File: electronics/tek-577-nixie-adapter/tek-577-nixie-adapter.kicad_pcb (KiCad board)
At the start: 2 copper layers, 31.7 x 61 mm, 6 parts, among them J1 C, J2 Conn_01x11_Socket, J3 E

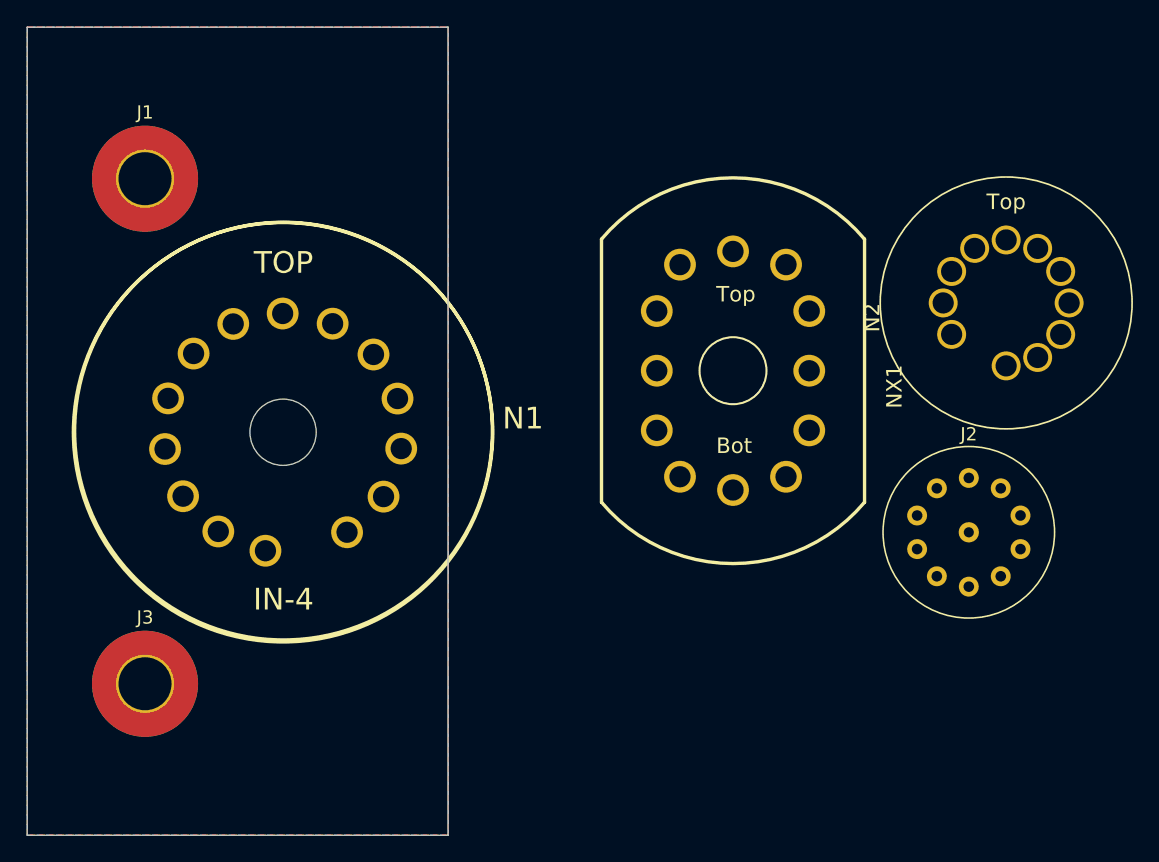
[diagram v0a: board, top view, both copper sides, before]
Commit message: board design done
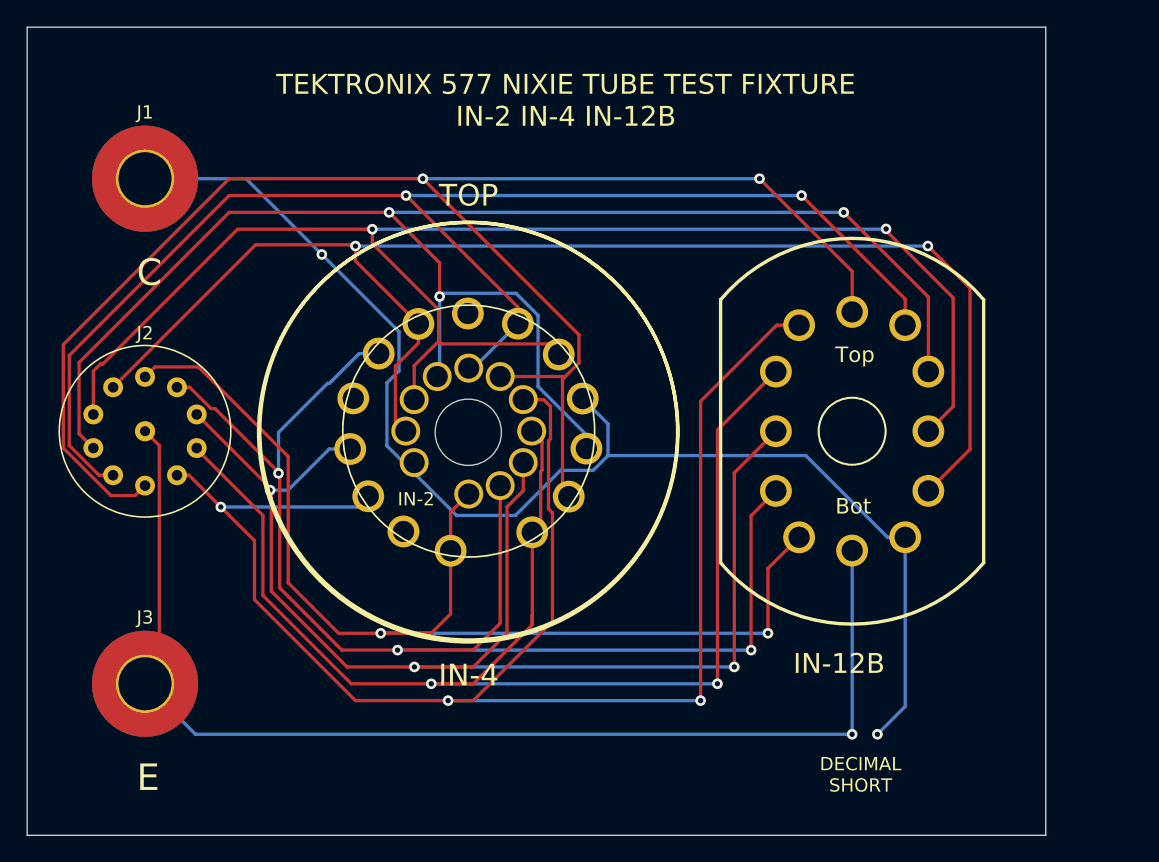
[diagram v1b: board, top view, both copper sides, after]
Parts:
- moved J2 62.6 mm to (134.6, 94.0)
- moved N2 41.7 mm to (159.0, 94.0)
- moved N1 14.0 mm to (159.0, 94.0)
- moved NX1 10.1 mm to (188.0, 94.0)
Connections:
- NX1 pad LHDP: unconnected-(NX1-PadLHDP) -> /E
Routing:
- net /5: track 0.00 -> 122.0 mm, vias 0 -> 3
- net /6: track 0.00 -> 120.9 mm, vias 0 -> 2
- net /8: track 0.00 -> 117.7 mm, vias 0 -> 3
- net /9: track 0.00 -> 110.8 mm, vias 0 -> 2
- net /0: track 0.00 -> 104.0 mm, vias 0 -> 2
- net /7: track 0.00 -> 102.5 mm, vias 0 -> 2
- net /2: track 0.00 -> 101.4 mm, vias 0 -> 3
- net /4: track 0.00 -> 101.0 mm, vias 0 -> 2
- net /3: track 0.00 -> 100.8 mm, vias 0 -> 3
- net /C: track 0.00 -> 99.9 mm, vias 0 -> 2
- net /E: track 0.00 -> 88.7 mm, vias 0 -> 1
- net /1: track 0.00 -> 84.9 mm, vias 0 -> 2
- removed copper zone on B.Cu, net (none)
- removed copper zone on F.Cu, net (none)
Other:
- board size 31.7 x 61 mm -> 76.8 x 61 mm
- board text added: "C"
- board text added: "DECIMAL SHORT"
- board text added: "E"
- board text added: "IN-12B"
- board text added: "IN-2"
- board text added: "TEKTRONIX 577 NIXIE TUBE TEST FIXTURE IN-2 IN-4 IN-12B"

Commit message: routing improvements
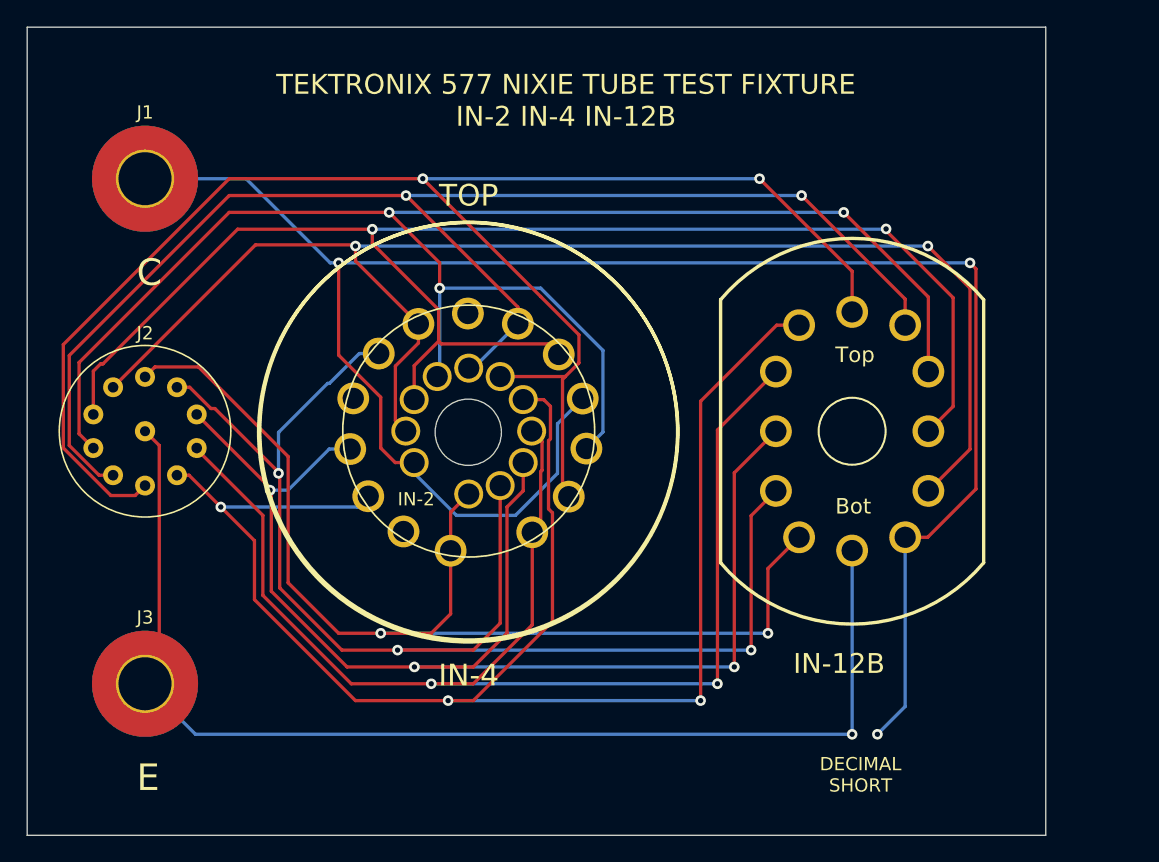
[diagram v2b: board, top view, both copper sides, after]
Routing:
- net /C: track 99.9 -> 143.6 mm, vias 2 -> 3
- net /8: track 117.7 -> 120.2 mm
- net /4: track 101.0 -> 100.3 mm
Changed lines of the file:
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@@
     (effects (font (size 2 2) (thickness 0.15)) (justify left bottom))
   )
+  (segment (start 152.4 95.25) (end 153.493357 96.343357) (width 0.25) (layer "F.Cu") (net 1))
+  (segment (start 149.225 88.239915) (end 152.4 91.414915) (width 0.25) (layer "F.Cu") (net 1))
+  (segment (start 196.85 81.28) (end 197.3 81.73) (width 0.25) (layer "F.Cu") (net 1))
+  (segment (start 153.493357 96.343357) (end 154.92327 96.343357) (width 0.25) (layer "F.Cu") (net 1))
+  (segment (start 149.225 81.28) (end 149.225 88.239915) (width 0.25) (layer "F.Cu") (net 1))
+  (segment (start 193.657056 101.98) (end 191.96 101.98) (width 0.25) (layer "F.Cu") (net 1))
+  (segment (start 197.3 98.337056) (end 193.657056 101.98) (width 0.25) (layer "F.Cu") (net 1))
+  (segment (start 197.3 81.73) (end 197.3 98.337056) (width 0.25) (layer "F.Cu") (net 1))
+  (segment (start 152.4 91.414915) (end 152.4 95.25) (width 0.25) (layer "F.Cu") (net 1))
   (via (at 189.865 116.84) (size 0.8) (drill 0.4) (layers "F.Cu" "B.Cu") (net 1))
-  (via (at 147.955 80.645) (size 0.8) (drill 0.4) (layers "F.Cu" "B.Cu") (net 1))
+  (via (at 149.225 81.28) (size 0.8) (drill 0.4) (layers "F.Cu" "B.Cu") (net 1))
+  (via (at 196.85 81.28) (size 0.8) (drill 0.4) (layers "F.Cu" "B.Cu") (net 1))
   (segment (start 191.96 114.745) (end 189.865 116.84) (width 0.25) (layer "B.Cu") (net 1))
+  (segment (start 154.92327 96.343357) (end 154.92327 97.13827) (width 0.25) (layer "B.Cu") (net 1))
+  (segment (start 165.735 93.417085) (end 167.637403 91.514682) (width 0.25) (layer "B.Cu") (net 1))
+  (segment (start 149.225 81.28) (end 148.59 81.28) (width 0.25) (layer "B.Cu") (net 1))
+  (segment (start 162.56 100.33) (end 165.735 97.155) (width 0.25) (layer "B.Cu") (net 1))
+  (segment (start 191.96 101.98) (end 191.96 114.745) (width 0.25) (layer "B.Cu") (net 1))
   (segment (start 154.92327 97.13827) (end 158.115 100.33) (width 0.25) (layer "B.Cu") (net 1))
-  (segment (start 153.778082 89.426918) (end 152.869716 90.335284) (width 0.25) (layer "B.Cu") (net 1))
-  (segment (start 147.955 80.645) (end 153.778082 86.468082) (width 0.25) (layer "B.Cu") (net 1))
-  (segment (start 162.56 100.33) (end 165.959619 96.930381) (width 0.25) (layer "B.Cu") (net 1))
-  (segment (start 169.545 95.816308) (end 169.545 93.422279) (width 0.25) (layer "B.Cu") (net 1))
-  (segment (start 154.92327 96.343357) (end 154.92327 97.13827) (width 0.25) (layer "B.Cu") (net 1))
-  (segment (start 154.128357 96.343357) (end 154.92327 96.343357) (width 0.25) (layer "B.Cu") (net 1))
-  (segment (start 142.24 74.93) (end 147.955 80.645) (width 0.25) (layer "B.Cu") (net 1))
-  (segment (start 169.545 95.816308) (end 184.469646 95.816308) (width 0.25) (layer "B.Cu") (net 1))
+  (segment (start 165.735 97.155) (end 165.735 93.417085) (width 0.25) (layer "B.Cu") (net 1))
   (segment (start 158.115 100.33) (end 162.56 100.33) (width 0.25) (layer "B.Cu") (net 1))
-  (segment (start 169.545 93.422279) (end 167.637403 91.514682) (width 0.25) (layer "B.Cu") (net 1))
-  (segment (start 168.430927 96.930381) (end 169.545 95.816308) (width 0.25) (layer "B.Cu") (net 1))
-  (segment (start 152.869716 95.084716) (end 154.128357 96.343357) (width 0.25) (layer "B.Cu") (net 1))
-  (segment (start 191.96 101.98) (end 191.96 114.745) (width 0.25) (layer "B.Cu") (net 1))
-  (segment (start 134.62 74.93) (end 142.24 74.93) (width 0.25) (layer "B.Cu") (net 1))
-  (segment (start 153.778082 86.468082) (end 153.778082 89.426918) (width 0.25) (layer "B.Cu") (net 1))
-  (segment (start 184.469646 95.816308) (end 190.633338 101.98) (width 0.25) (layer "B.Cu") (net 1))
-  (segment (start 165.959619 96.930381) (end 168.430927 96.930381) (width 0.25) (layer "B.Cu") (net 1))
-  (segment (start 152.869716 90.335284) (end 152.869716 95.084716) (width 0.25) (layer "B.Cu") (net 1))
-  (segment (start 190.633338 101.98) (end 191.96 101.98) (width 0.25) (layer "B.Cu") (net 1))
+  (segment (start 149.225 81.28) (end 196.85 81.28) (width 0.25) (layer "B.Cu") (net 1))
+  (segment (start 148.59 81.28) (end 142.24 74.93) (width 0.25) (layer "B.Cu") (net 1))
+  (segment (start 142.24 74.93) (end 134.62 74.93) (width 0.25) (layer "B.Cu") (net 1))
   (segment (start 135.695 95.055) (end 134.62 93.98) (width 0.25) (layer "F.Cu") (net 2))
   (segment (start 134.62 113.03) (end 135.695 111.955) (width 0.25) (layer "F.Cu") (net 2))
@@
   (segment (start 177.8 93.89) (end 182.21 89.48) (width 0.25) (layer "F.Cu") (net 6))
   (segment (start 164.567362 96.930381) (end 164.567362 94.749303) (width 0.25) (layer "F.Cu") (net 6))
-  (segment (start 163.83 108.585) (end 163.83 107.86) (width 0.25) (layer "F.Cu") (net 6))
   (segment (start 159.385 113.03) (end 163.83 108.585) (width 0.25) (layer "F.Cu") (net 6))
   (segment (start 143.51 100.33) (end 138.519331 95.339331) (width 0.25) (layer "F.Cu") (net 6))
@@
   (segment (start 159.39156 89.218657) (end 159.036716 89.218657) (width 0.25) (layer "B.Cu") (net 9))
   (segment (start 193.71 83.855) (end 193.71 89.48) (width 0.25) (layer "F.Cu") (net 10))
+  (segment (start 156.845 81.28) (end 153.035 77.47) (width 0.25) (layer "F.Cu") (net 10))
   (segment (start 187.325 77.47) (end 193.71 83.855) (width 0.25) (layer "F.Cu") (net 10))
   (segment (start 129.645669 88.792935) (end 129.645669 94.171969) (width 0.25) (layer "F.Cu") (net 10))
@@
   (segment (start 153.035 77.47) (end 140.968604 77.47) (width 0.25) (layer "F.Cu") (net 10))
   (segment (start 140.968604 77.47) (end 129.645669 88.792935) (width 0.25) (layer "F.Cu") (net 10))
-  (segment (start 156.845 81.28) (end 156.845 83.82) (width 0.25) (layer "F.Cu") (net 10))
-  (segment (start 153.035 77.47) (end 156.845 81.28) (width 0.25) (layer "F.Cu") (net 10))
+  (segment (start 156.845 83.185) (end 156.845 81.28) (width 0.25) (layer "F.Cu") (net 10))
   (via (at 187.325 77.47) (size 0.8) (drill 0.4) (layers "F.Cu" "B.Cu") (net 10))
   (via (at 153.035 77.47) (size 0.8) (drill 0.4) (layers "F.Cu" "B.Cu") (net 10))
-  (via (at 156.845 83.82) (size 0.8) (drill 0.4) (layers "F.Cu" "B.Cu") (net 10))
-  (segment (start 162.608478 83.574807) (end 164.268606 85.234935) (width 0.25) (layer "B.Cu") (net 10))
-  (segment (start 164.268606 85.234935) (end 164.268606 90.608606) (width 0.25) (layer "B.Cu") (net 10))
-  (segment (start 164.268606 90.608606) (end 167.914616 94.254616) (width 0.25) (layer "B.Cu") (net 10))
-  (segment (start 156.845 83.82) (end 156.845 89.671827) (width 0.25) (layer "B.Cu") (net 10))
-  (segment (start 167.914616 94.254616) (end 167.914616 95.290016) (width 0.25) (layer "B.Cu") (net 10))
+  (via (at 156.845 83.185) (size 0.8) (drill 0.4) (layers "F.Cu" "B.Cu") (net 10))
+  (segment (start 156.845 83.185) (end 164.465 83.185) (width 0.25) (layer "B.Cu") (net 10))
+  (segment (start 156.845 83.185) (end 156.845 89.671827) (width 0.25) (layer "B.Cu") (net 10))
   (segment (start 156.845 89.671827) (end 156.661816 89.855011) (width 0.25) (layer "B.Cu") (net 10))
+  (segment (start 164.465 83.185) (end 169.162403 87.882403) (width 0.25) (layer "B.Cu") (net 10))
   (segment (start 153.035 77.47) (end 187.325 77.47) (width 0.25) (layer "B.Cu") (net 10))
-  (segment (start 156.845 83.82) (end 157.090193 83.574807) (width 0.25) (layer "B.Cu") (net 10))
-  (segment (start 157.090193 83.574807) (end 162.608478 83.574807) (width 0.25) (layer "B.Cu") (net 10))
+  (segment (start 169.162403 87.882403) (end 169.162403 94.042229) (width 0.25) (layer "B.Cu") (net 10))
+  (segment (start 169.162403 94.042229) (end 167.914616 95.290016) (width 0.25) (layer "B.Cu") (net 10))
   (segment (start 131.266338 88.9) (end 130.720669 89.445669) (width 0.25) (layer "F.Cu") (net 11))
   (segment (start 151.765 78.74) (end 141.605 78.74) (width 0.25) (layer "F.Cu") (net 11))
